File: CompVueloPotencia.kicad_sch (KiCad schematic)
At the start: 2 parts, among them U1 ESP32-S3-WROOM-1

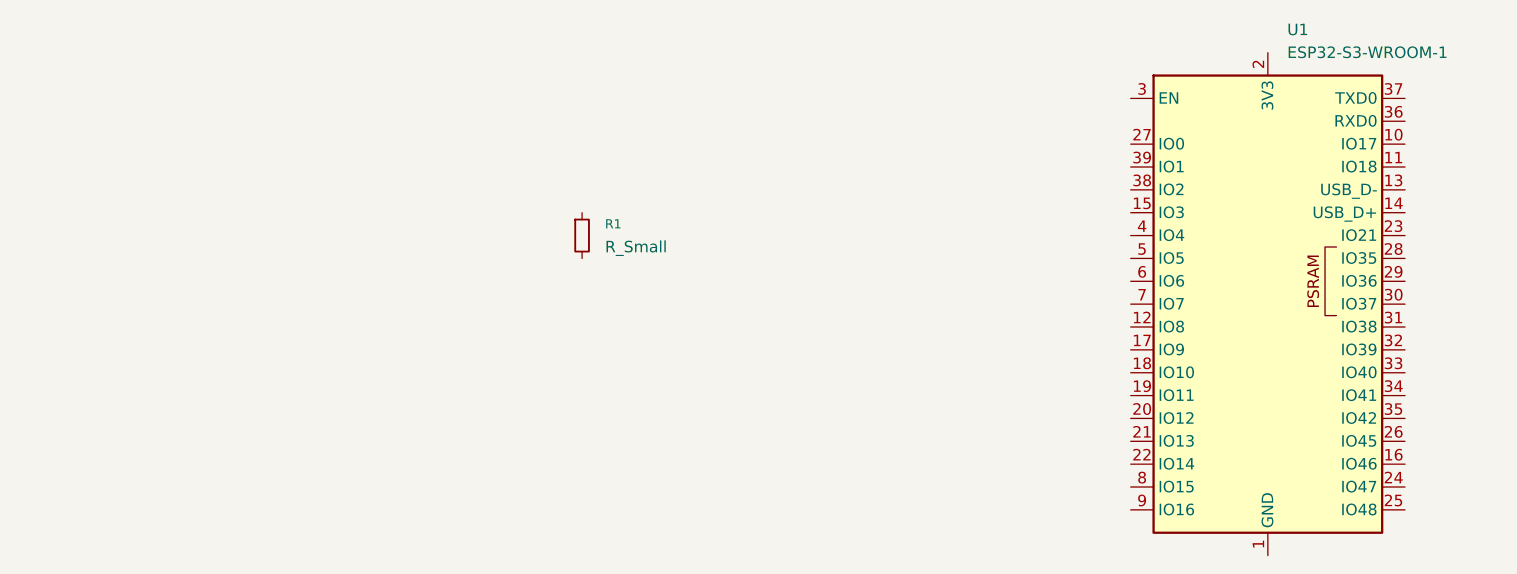
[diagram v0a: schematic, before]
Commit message: another test of updates
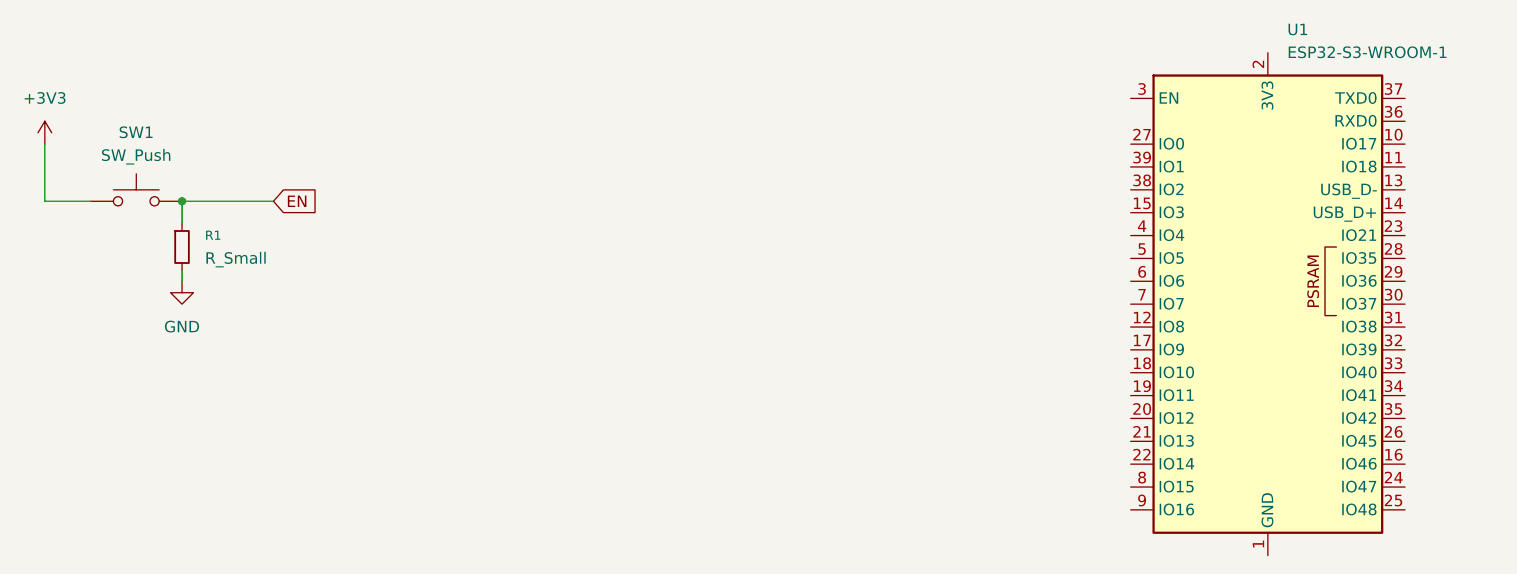
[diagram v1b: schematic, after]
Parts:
- added SW1: SW_Push, symbol Switch:SW_Push
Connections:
- net EN: now reaches R1.1
- net EN: now also SW1.2
- net GND: now reaches R1.2
- new net +3V3: SW1.1
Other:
- moved on the sheet: R1
